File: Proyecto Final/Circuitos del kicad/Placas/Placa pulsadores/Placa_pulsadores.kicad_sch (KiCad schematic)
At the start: 10 parts, among them J1 Conn_02x06_Odd_Even, SW1 SW_Push, SW2 SW_Push, SW3 SW_Push, SW4 SW_Push

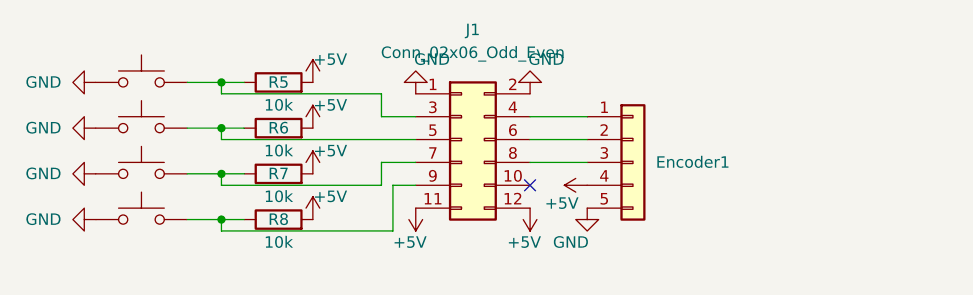
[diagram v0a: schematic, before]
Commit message: chc
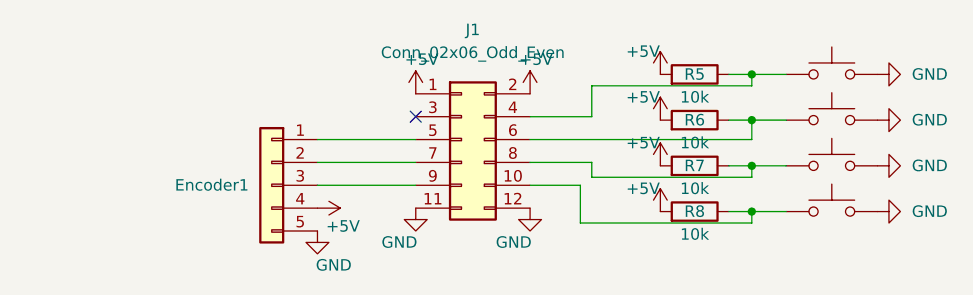
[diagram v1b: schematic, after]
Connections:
- net +5V: now also J1.1 (Pin_1), J1.2 (Pin_2); no longer J1.11 (Pin_11), J1.12 (Pin_12)
- net GND: now also J1.11 (Pin_11), J1.12 (Pin_12); no longer J1.1 (Pin_1), J1.2 (Pin_2)
- net at R7.1, SW2.2: now also J1.8 (Pin_8); no longer J1.7 (Pin_7)
- net at J1.10 (Pin_10): now also R8.1, SW1.2
- net at R5.1, SW4.2: now also J1.4 (Pin_4); no longer J1.3 (Pin_3)
- net at Encoder1.1 (Pin_1): now also J1.5 (Pin_5); no longer J1.4 (Pin_4)
- net at R6.1, SW3.2: now also J1.6 (Pin_6); no longer J1.5 (Pin_5)
- net at Encoder1.2 (Pin_2): now also J1.7 (Pin_7); no longer J1.6 (Pin_6)
- net at Encoder1.3 (Pin_3): now also J1.9 (Pin_9); no longer J1.8 (Pin_8)
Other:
- moved on the sheet: Encoder1, R5, R6, R7, R8
